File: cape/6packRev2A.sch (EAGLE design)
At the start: 16 parts

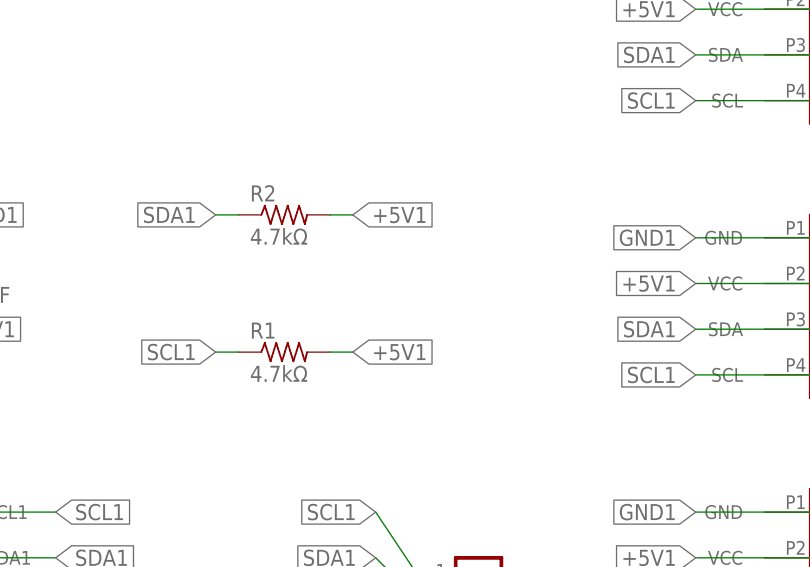
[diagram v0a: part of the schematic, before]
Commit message: Revert "Update 6Pack 2A"
This reverts commit 827b5304b12bda17fe1987ea76be93996f945791.
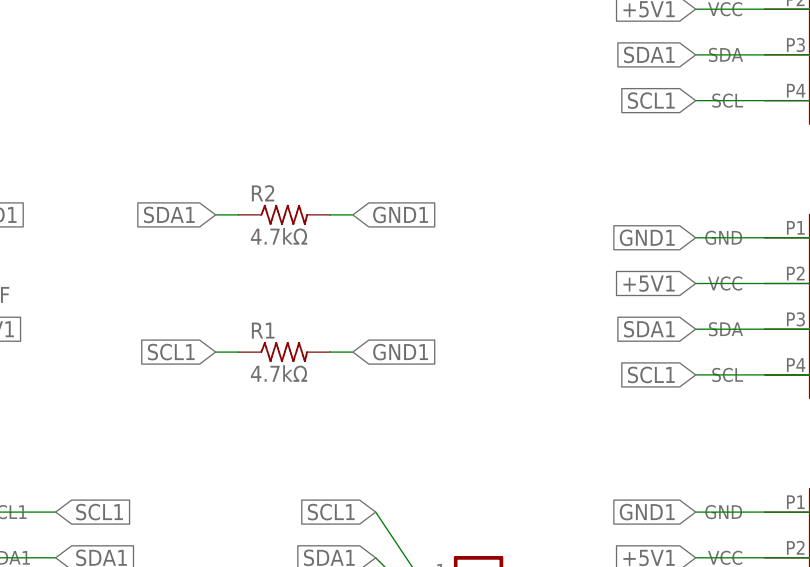
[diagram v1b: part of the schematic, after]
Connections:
- net +5V1: no longer R1.2, R2.2
- net GND1: now also R1.2, R2.2
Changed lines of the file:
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@@
 <label x="144.78" y="48.26" size="1.778" layer="95" rot="R180" xref="yes"/>
-</segment>
-<segment>
-<pinref part="R2" gate="G$1" pin="2"/>
-<wire x1="139.7" y1="91.44" x2="142.24" y2="91.44" width="0.1524" layer="91"/>
-<label x="142.24" y="91.44" size="1.778" layer="95" xref="yes"/>
-</segment>
-<segment>
-<pinref part="R1" gate="G$1" pin="2"/>
-<wire x1="139.7" y1="76.2" x2="142.24" y2="76.2" width="0.1524" layer="91"/>
-<label x="142.24" y="76.2" size="1.778" layer="95" xref="yes"/>
 </segment>
 </net>
@@
 <label x="144.78" y="43.18" size="1.778" layer="95" rot="R180" xref="yes"/>
 </segment>
+<segment>
+<pinref part="R1" gate="G$1" pin="2"/>
+<wire x1="139.7" y1="76.2" x2="142.24" y2="76.2" width="0.1524" layer="91"/>
+<label x="142.24" y="76.2" size="1.778" layer="95" xref="yes"/>
+</segment>
+<segment>
+<pinref part="R2" gate="G$1" pin="2"/>
+<wire x1="139.7" y1="91.44" x2="142.24" y2="91.44" width="0.1524" layer="91"/>
+<label x="142.24" y="91.44" size="1.778" layer="95" xref="yes"/>
+</segment>
 </net>

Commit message: Update 6Pack 2A
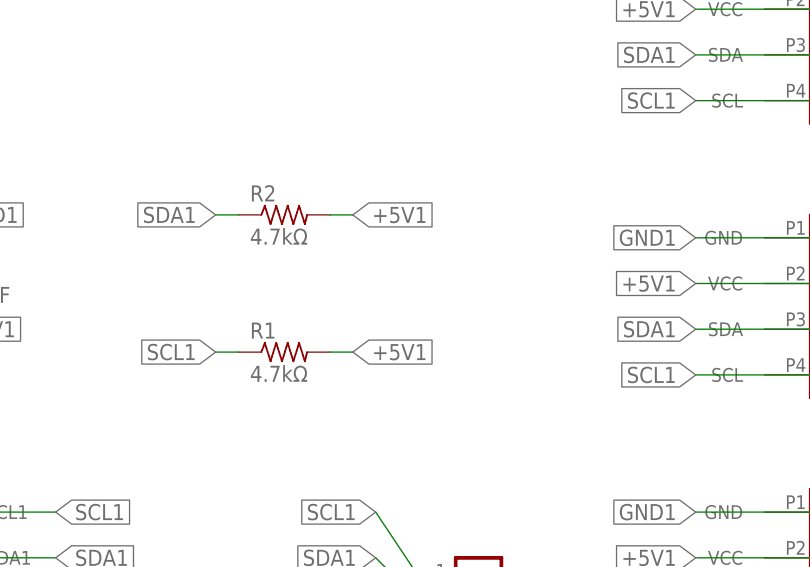
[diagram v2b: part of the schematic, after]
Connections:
- net +5V1: now also R1.2, R2.2
- net GND1: no longer R1.2, R2.2
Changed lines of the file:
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@@
 <label x="144.78" y="48.26" size="1.778" layer="95" rot="R180" xref="yes"/>
+</segment>
+<segment>
+<pinref part="R2" gate="G$1" pin="2"/>
+<wire x1="139.7" y1="91.44" x2="142.24" y2="91.44" width="0.1524" layer="91"/>
+<label x="142.24" y="91.44" size="1.778" layer="95" xref="yes"/>
+</segment>
+<segment>
+<pinref part="R1" gate="G$1" pin="2"/>
+<wire x1="139.7" y1="76.2" x2="142.24" y2="76.2" width="0.1524" layer="91"/>
+<label x="142.24" y="76.2" size="1.778" layer="95" xref="yes"/>
 </segment>
 </net>
@@
 <label x="144.78" y="43.18" size="1.778" layer="95" rot="R180" xref="yes"/>
 </segment>
-<segment>
-<pinref part="R1" gate="G$1" pin="2"/>
-<wire x1="139.7" y1="76.2" x2="142.24" y2="76.2" width="0.1524" layer="91"/>
-<label x="142.24" y="76.2" size="1.778" layer="95" xref="yes"/>
-</segment>
-<segment>
-<pinref part="R2" gate="G$1" pin="2"/>
-<wire x1="139.7" y1="91.44" x2="142.24" y2="91.44" width="0.1524" layer="91"/>
-<label x="142.24" y="91.44" size="1.778" layer="95" xref="yes"/>
-</segment>
 </net>
